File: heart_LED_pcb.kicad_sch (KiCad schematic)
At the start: 6 parts, among them J1 USB_C_2.0_16P, U1 ESP32-C3, U2 AMS1117-3.3

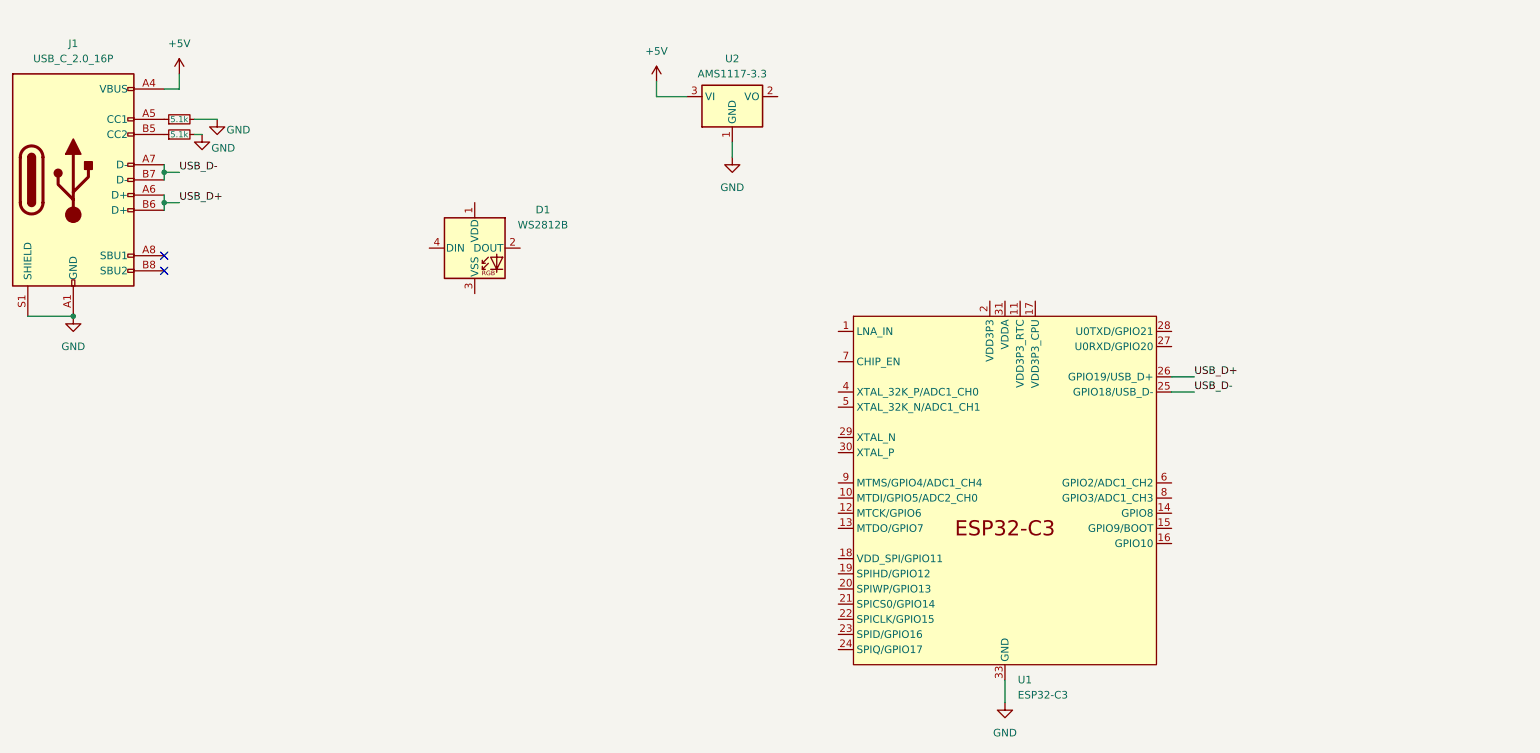
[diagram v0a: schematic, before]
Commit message: Updated schematic
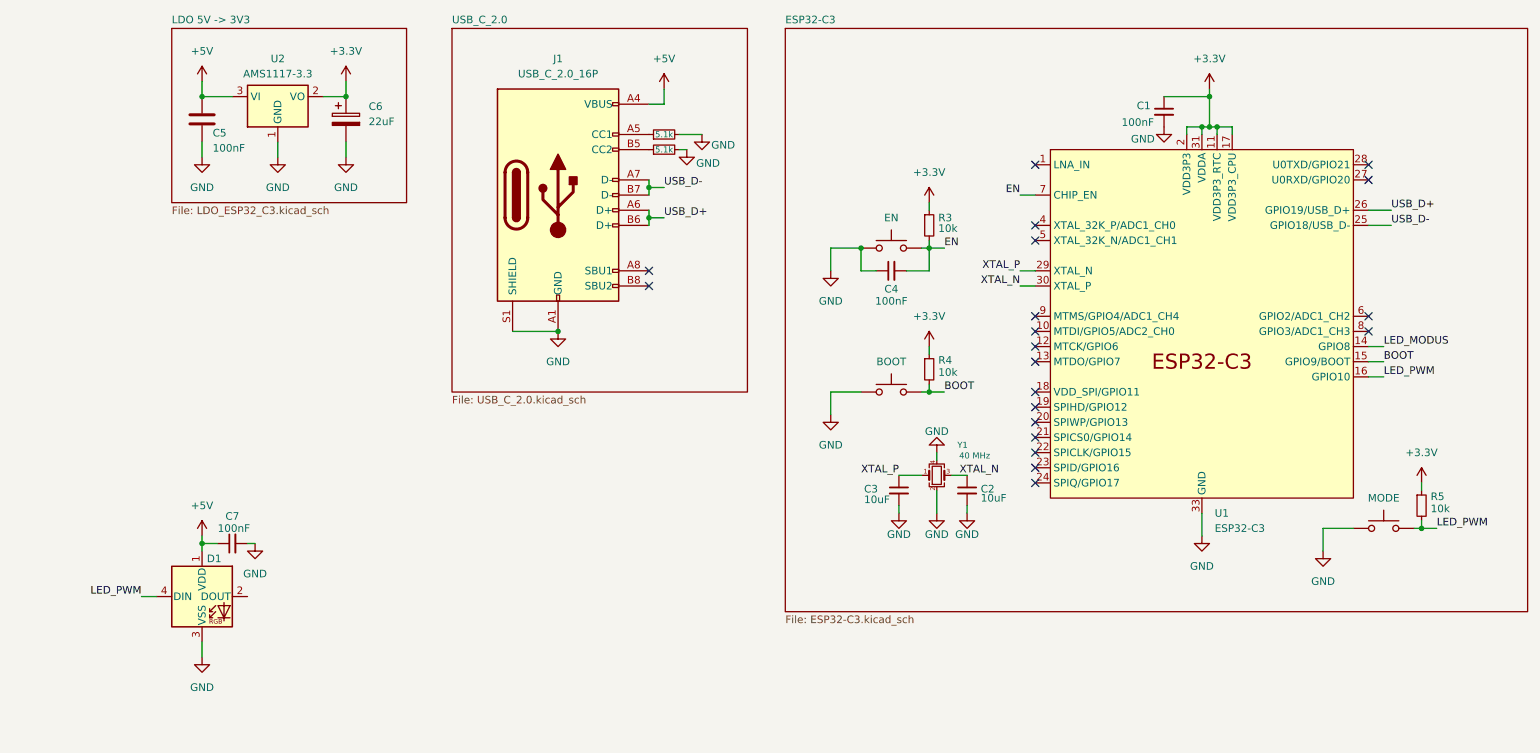
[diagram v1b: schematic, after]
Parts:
- added C1: 100nF, Capacitor_SMD:CP_Elec_CAP-XX_DMF3Zxxxxxxxx3D, symbol Device:C_Small
- added C2, C3: 10uF, symbol Device:C_Small
- added C4: 100nF, symbol Device:C_Small
- added C5: 100nF, Capacitor_SMD:C_0402_1005Metric, symbol Device:C
- added C6: 22uF, Capacitor_Tantalum_SMD:CP_EIA-3216-18_Kemet-A, symbol Device:C_Polarized
- added C7: 100nF, Capacitor_SMD:C_0201_0603Metric, symbol Device:C_Small
- added R3, R4, R5: 10k, symbol Device:R_Small
- added SW1: EN, symbol Switch:SW_Push
- added SW2: BOOT, symbol Switch:SW_Push
- added SW3: MODE, symbol Switch:SW_Push
- added Y1: 40 MHz, Crystal:Crystal_SMD_TXC_7M-4Pin_3.2x2.5mm, symbol Device:Crystal_GND24_Small
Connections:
- net +5V: now also D1.1 (VDD), C5.1, C7.1
- net GND: now also D1.3 (VSS), C1.2, C2.2, C3.2, C4.1, C5.2, C6.2, C7.2, SW1.1, SW2.1, SW3.1, Y1.2, Y1.4
- net +3.3V: now reaches U1.11 (VDD3P3_RTC)
- net +3.3V: now also U1.17 (VDD3P3_CPU), U1.2 (VDD3P3), U1.3 (VDD3P3), U1.31 (VDDA), U1.32 (VDDA), U2.2 (VO), C1.1, C6.1, R3.1, R4.1, R5.1
- net LED_MODUS: now reaches U1.14 (GPIO8)
- net BOOT: now reaches U1.15 (GPIO9/BOOT)
- net BOOT: now also R4.2, SW2.2
- net LED_PWM: now reaches U1.16 (GPIO10)
- net LED_PWM: now also D1.4 (DIN), R5.2, SW3.2
- net XTAL_P: now reaches U1.29 (XTAL_N)
- net XTAL_P: now also C3.1, Y1.1
- net XTAL_N: now reaches U1.30 (XTAL_P)
- net XTAL_N: now also C2.1, Y1.3
- net EN: now reaches U1.7 (CHIP_EN)
- net EN: now also C4.2, R3.2, SW1.2
- no-connect marks 2 -> 20
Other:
- added sheet ESP32-C3 (ESP32-C3.kicad_sch)
- added sheet LDO 5V -> 3V3 (LDO_ESP32_C3.kicad_sch)
- added sheet USB_C_2.0 (USB_C_2.0.kicad_sch)
- moved on the sheet: D1, J1, U1, U2
